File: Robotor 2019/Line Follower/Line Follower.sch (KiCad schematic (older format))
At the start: 96 parts, among them J1 Conn_01x03_Male, J2 Conn_01x04_Female, J3 USB_B_Mini, J4 Conn_01x03_Female, J5 Conn_01x03_Female, J7 Conn_01x03_Female, J8 Conn_01x03_Female, M1 Motor_DC, M2 Motor_DC, U1 AMS1117-3V3, U10 ITR8307, U11 ITR8307, U12 ITR8307, U13 ITR8307, U14 ITR8307, U15 ITR8307, U3 AMS1117-5.0, U4 STM32F103C8Tx, U5 ITR8307, U6 L298P, U7 ITR8307, U8 ITR8307, U9 ITR8307, Y1 32.768Khz, Y2 8Mhz

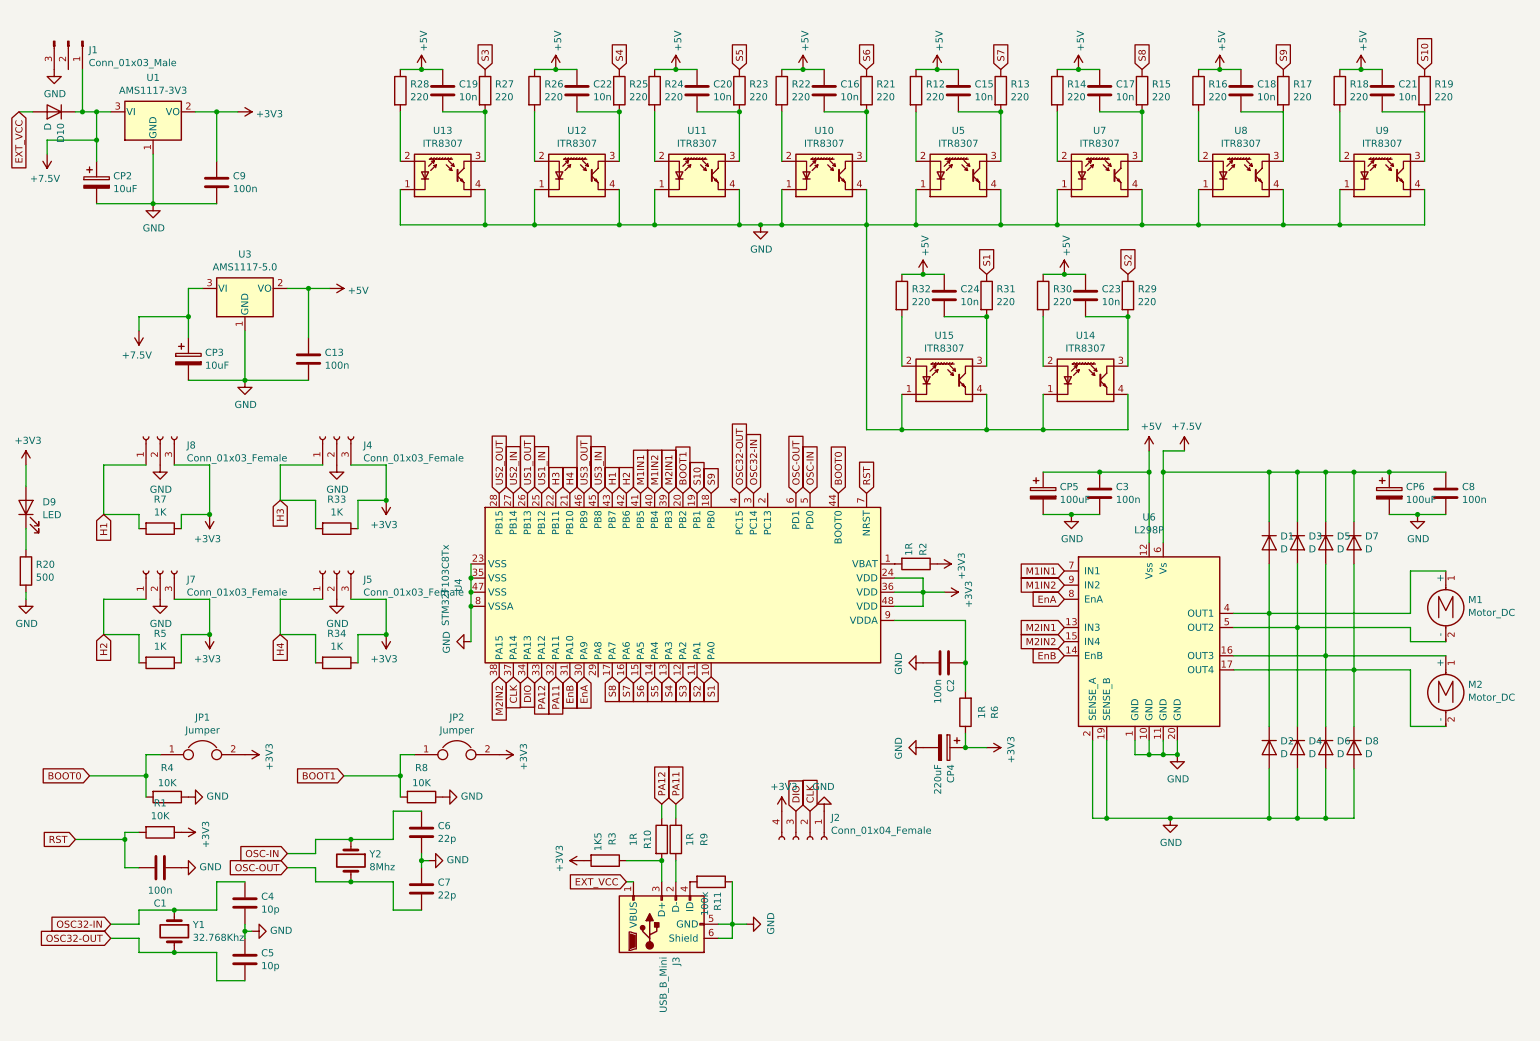
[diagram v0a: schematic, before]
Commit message: Line Follower robot electric schematic and PCB.
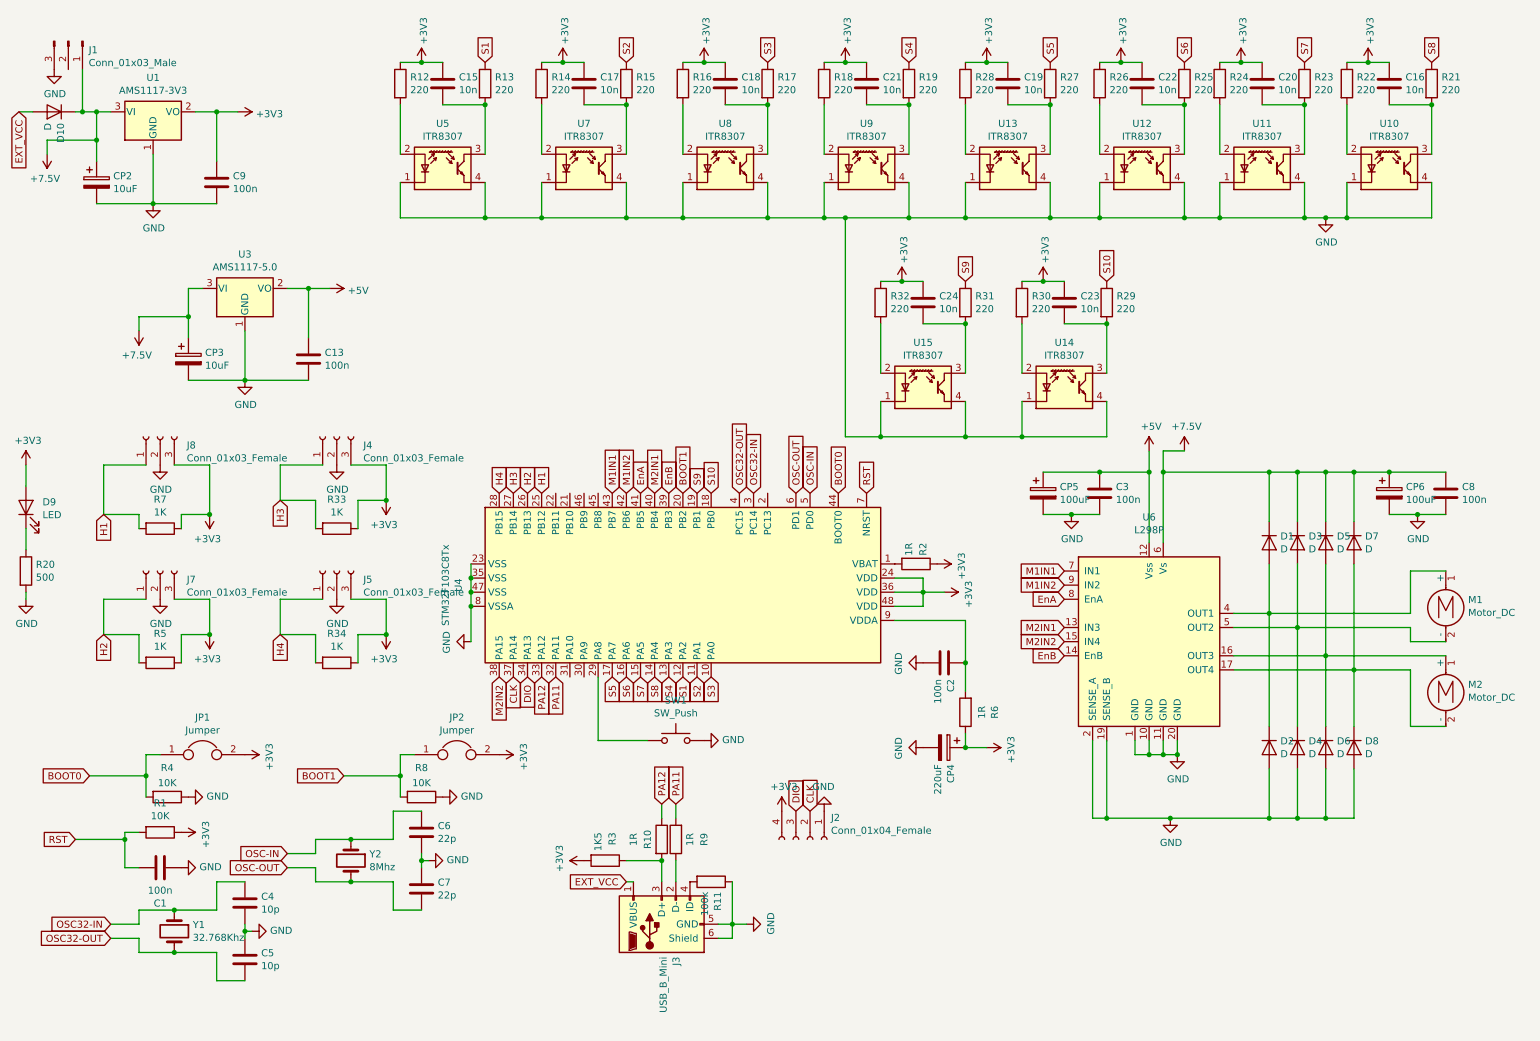
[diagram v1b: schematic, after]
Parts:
- added SW1: SW_Push, Button_Switch_SMD:SW_Push_1P1T_NO_6x6mm_H9.5mm, symbol Switch:SW_Push
- R12, R13, R14, R15, R16, R17, R18, R19, R21, R22, R23, R24, R25, R26, R27, R28, R29, R30, R31, R32: footprint Resistor_SMD:R_0805_2012Metric_Pad1.15x1.40mm_HandSolder -> Resistor_SMD:R_1206_3216Metric_Pad1.42x1.75mm_HandSolder
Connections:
- net US1_IN is gone; now on net H1: U4.25 (PB12)
- net US1_OUT is gone; now on net H2: U4.26 (PB13)
- net US2_IN is gone; now on net H3: U4.27 (PB14)
- net US2_OUT is gone; now on net H4: U4.28 (PB15)
- net +3V3: now also C15.1, C16.1, C17.1, C18.1, C19.1, C20.1, C21.1, C22.1, C23.1, C24.1, R12.1, R14.1, R16.1, R18.1, R22.1, R24.1, R26.1, R28.1, R30.1, R32.1
- net +5V: no longer C15.1, C16.1, C17.1, C18.1, C19.1, C20.1, C21.1, C22.1, C23.1, C24.1, R12.1, R14.1, R16.1, R18.1, R22.1, R24.1, R26.1, R28.1, R30.1, R32.1
- net EnA: now also U4.41 (PB5); no longer U4.30 (PA9)
- net EnB: now also U4.39 (PB3); no longer U4.31 (PA10)
- net GND: now also SW1.2
- net H1: no longer U4.43 (PB7)
- net H2: no longer U4.42 (PB6)
- net H3: no longer U4.22 (PB11)
- net H4: no longer U4.21 (PB10)
- net M1IN1: now also U4.43 (PB7); no longer U4.41 (PB5)
- net M1IN2: now also U4.42 (PB6); no longer U4.40 (PB4)
- net M2IN1: now also U4.40 (PB4); no longer U4.39 (PB3)
- net S1: now also R13.1, U4.12 (PA2); no longer R31.1, U4.10 (PA0)
- net S10: now also R29.1, U4.18 (PB0); no longer R19.1, U4.19 (PB1)
- net S2: now also R15.1; no longer R29.1
- net S3: now also R17.1, U4.10 (PA0); no longer R27.1, U4.12 (PA2)
- net S4: now also R19.1; no longer R25.1
- net S5: now also R27.1, U4.17 (PA7); no longer R23.1, U4.14 (PA4)
- net S6: now also R25.1, U4.16 (PA6); no longer R21.1, U4.15 (PA5)
- net S7: now also R23.1, U4.15 (PA5); no longer R13.1, U4.16 (PA6)
- net S8: now also R21.1, U4.14 (PA4); no longer R15.1, U4.17 (PA7)
- net S9: now also R31.1, U4.19 (PB1); no longer R17.1, U4.18 (PB0)
- net at U4.29 (PA8): now also SW1.1
- net US3_IN: no longer names the net of U4.45 (PB8)
- net US3_OUT: no longer names the net of U4.46 (PB9)
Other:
- moved on the sheet: C15, C16, C17, C18, C19, C20, C21, C22, C23, C24, R12, R13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
